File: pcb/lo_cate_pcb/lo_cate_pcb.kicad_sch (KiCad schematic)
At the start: 49 parts, among them J1 Conn_01x07_Pin, J2 690-005-299-043, J3 U.FL-R-SMT-110, SW1 MICRO_RESET, SW2 MICRO_ON, SW3 BUTTON1, SW4 BUTTON2, SW5 BUTTON3, U1 STM32F401RETx, U2 BMI323, U3 LED1, U4 LED2, U5 LED3, U6 RFM95W-868S2, U7 LDK320AM33R

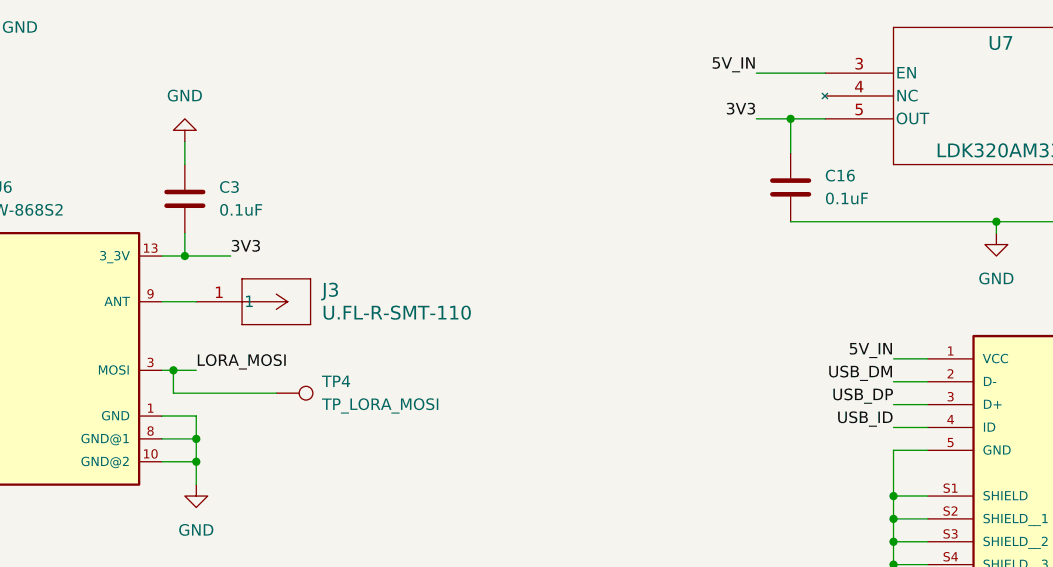
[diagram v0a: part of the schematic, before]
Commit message: Final PCB design done
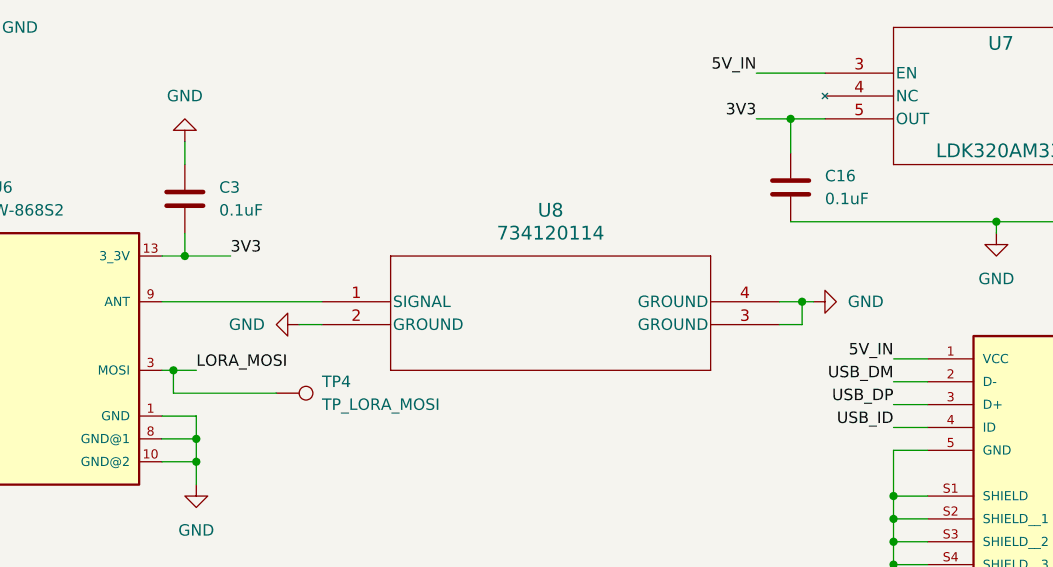
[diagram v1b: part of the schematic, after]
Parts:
- removed J3: U.FL-R-SMT-110, footprints:CONN1_UFL-R_HIR, symbol 2024-06-24_09-28-13:U.FL-R-SMT-110
- added U8: 734120114, footprints:73412-0114_MOL, symbol 2024-06-27_09-08-45:734120114
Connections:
- net GND: now also U8.2 (GROUND), U8.3 (GROUND), U8.4 (GROUND)
- net at U6.9 (ANT): now also U8.1 (SIGNAL)
